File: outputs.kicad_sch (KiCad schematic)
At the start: 22 parts, among them Q1 ISL9V3040D3ST, Q2 ISL9V3040D3ST, U2 VNLD5160TR-E, U3 VNLD5160TR-E, U4 VNLD5160TR-E, U5 TLE9201SGAUMA1, U6 VNLD5160TR-E

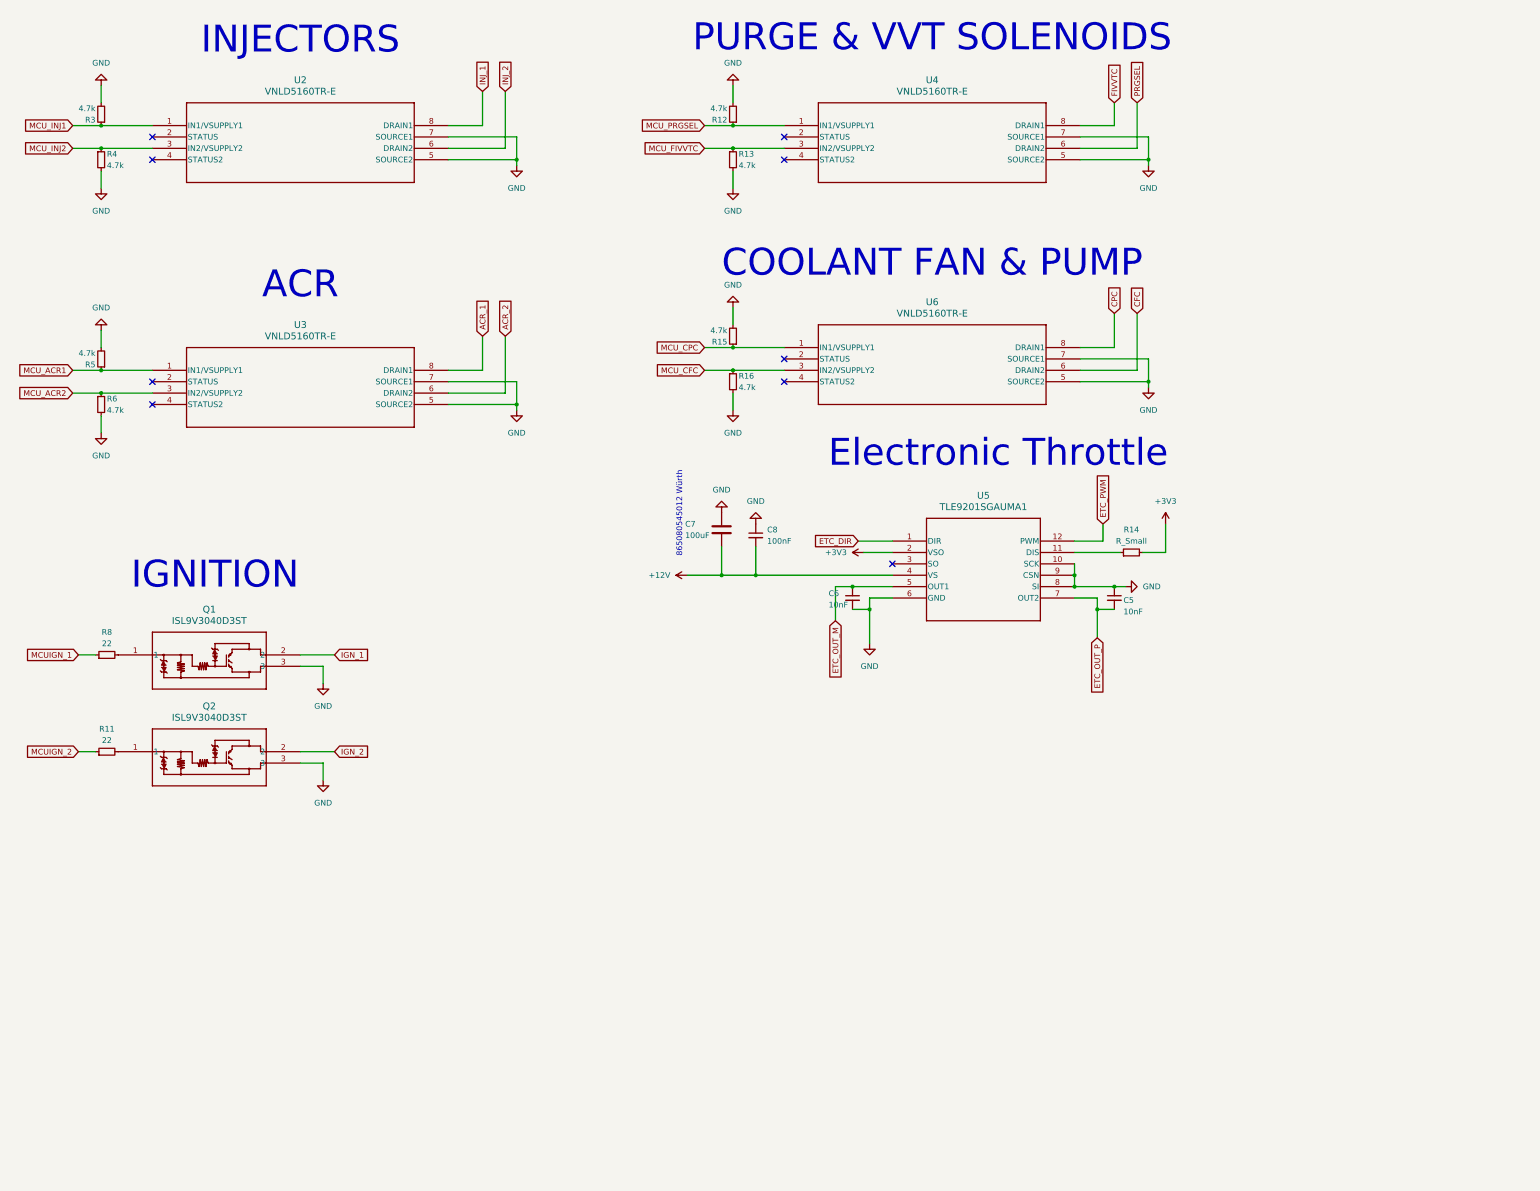
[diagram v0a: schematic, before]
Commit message: redone layout, possibly feature complete
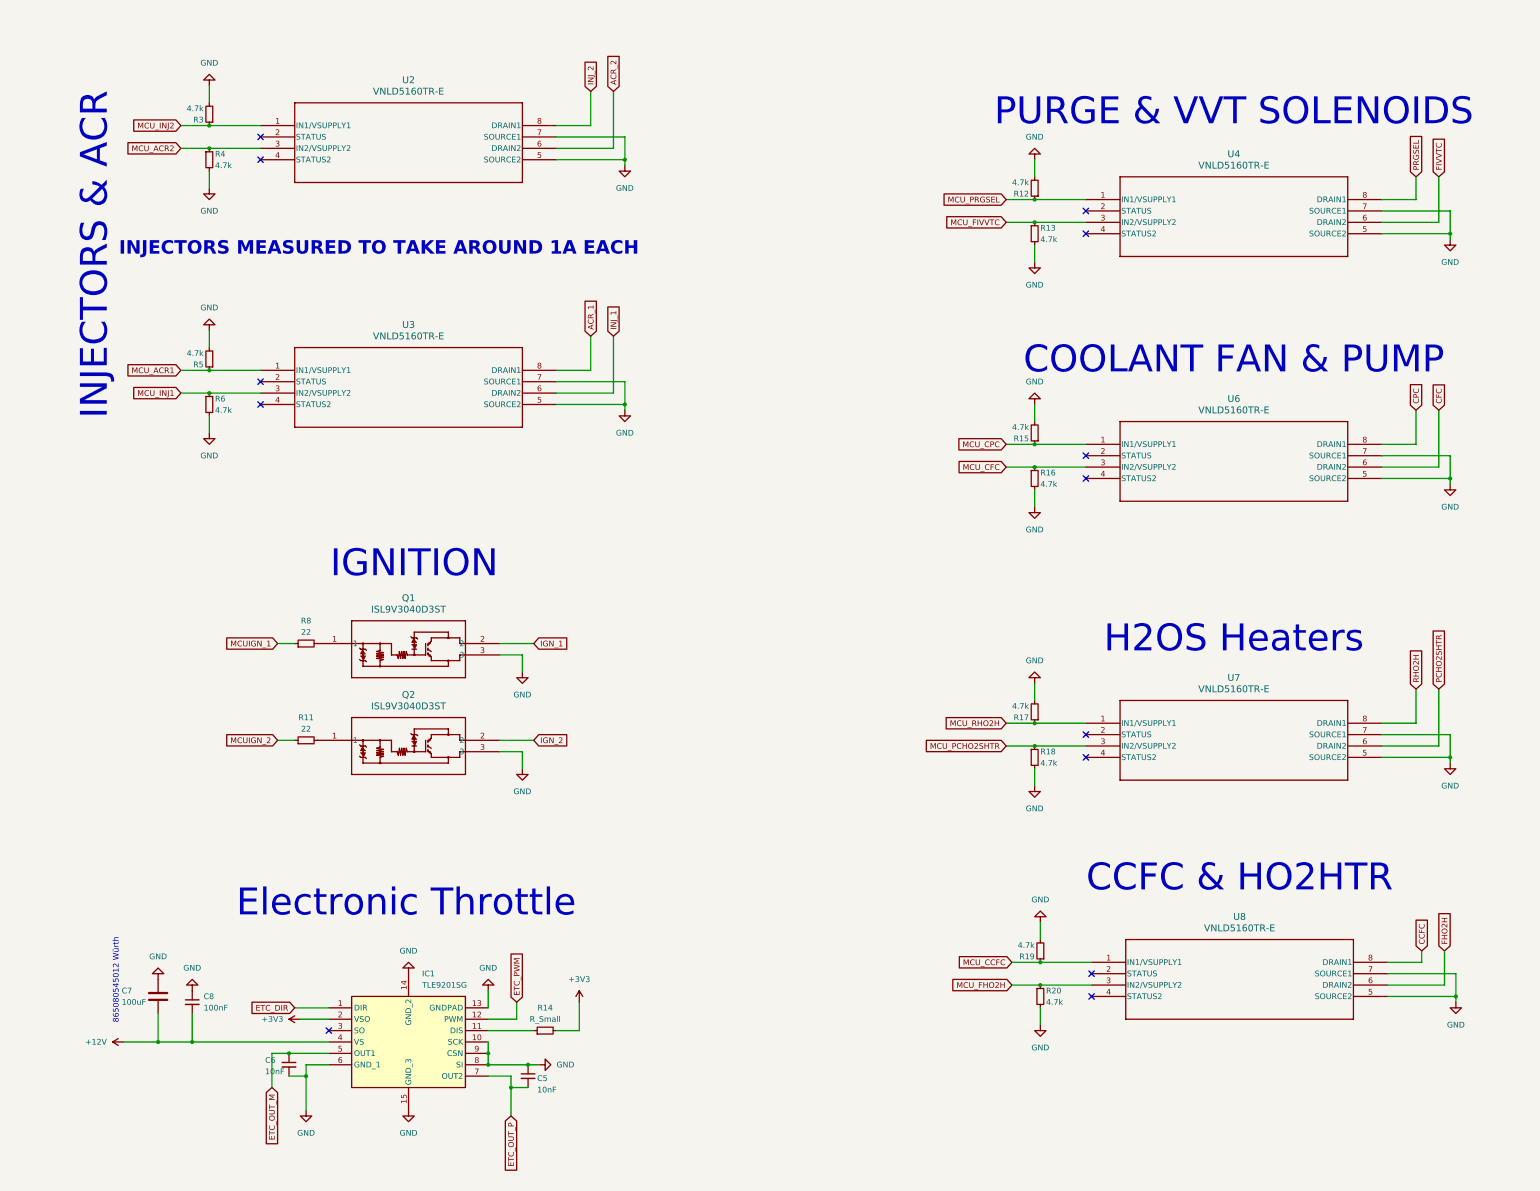
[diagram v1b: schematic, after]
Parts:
- removed U5: TLE9201SGAUMA1, TLE9201SG:TLE9201SGAUMA1_INF, symbol TLE9201SG:TLE9201SGAUMA1
- added IC1: TLE9201SG, TLE9201SG:TLE9201SG, symbol TLE9201SG:TLE9201SG
- added R17, R18, R19, R20: 4.7k, Resistor_SMD:R_0402_1005Metric, symbol Device:R_Small
- added U7, U8: VNLD5160TR-E, VNLD5160TR-E:SO_160TR-E_STM, symbol VNLD5160TR-E:VNLD5160TR-E
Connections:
- net +12V: now also IC1.4 (VS)
- net +3V3: now also IC1.2 (VSO)
- net ACR_2: now also U2.6 (DRAIN2); no longer U3.6 (DRAIN2)
- net ETC_DIR: now also IC1.1 (DIR)
- net ETC_OUT_M: now also IC1.5 (OUT1)
- net ETC_OUT_P: now also IC1.7 (OUT2)
- net ETC_PWM: now also IC1.12 (PWM)
- net FIVVTC: now also U4.6 (DRAIN2); no longer U4.8 (DRAIN1)
- net GND: now also IC1.10 (SCK), IC1.13 (GNDPAD), IC1.14 (GND_2), IC1.15 (GND_3), IC1.6 (GND_1), IC1.8 (SI), IC1.9 (CSN), R17.2, R18.2, R19.2, R20.2, U7.5 (SOURCE2), U7.7 (SOURCE1), U8.5 (SOURCE2), U8.7 (SOURCE1)
- net INJ_1: now also U3.6 (DRAIN2); no longer U2.8 (DRAIN1)
- net INJ_2: now also U2.8 (DRAIN1); no longer U2.6 (DRAIN2)
- net MCU_ACR2: now also R4.1, U2.3 (IN2/VSUPPLY2); no longer R6.1, U3.3 (IN2/VSUPPLY2)
- net MCU_INJ1: now also R6.1, U3.3 (IN2/VSUPPLY2); no longer R3.1, U2.1 (IN1/VSUPPLY1)
- net MCU_INJ2: now also R3.1, U2.1 (IN1/VSUPPLY1); no longer R4.1, U2.3 (IN2/VSUPPLY2)
- net PRGSEL: now also U4.8 (DRAIN1); no longer U4.6 (DRAIN2)
- net at R14.1: now also IC1.11 (DIS)
- new net CCFC: U8.8 (DRAIN1)
- new net FHO2H: U8.6 (DRAIN2)
- new net MCU_CCFC: R19.1, U8.1 (IN1/VSUPPLY1)
- new net MCU_FHO2H: R20.1, U8.3 (IN2/VSUPPLY2)
- new net MCU_PCHO2SHTR: R18.1, U7.3 (IN2/VSUPPLY2)
- new net MCU_RHO2H: R17.1, U7.1 (IN1/VSUPPLY1)
- new net PCHO2SHTR: U7.6 (DRAIN2)
- new net RHO2H: U7.8 (DRAIN1)
- no-connect marks 9 -> 13
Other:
- note added: "CCFC & HO2HTR"
- note added: "H2OS Heaters"
- note added: "INJECTORS & ACR"
- note added: "INJECTORS MEASURED TO TAKE AROUND 1A EACH"
- note removed: "ACR"
- note removed: "INJECTORS"
- moved on the sheet: Q1, Q2, R11, R12, R13, R15, R16, R3, R4, R5, R6, R8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
